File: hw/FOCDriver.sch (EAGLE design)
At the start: 95 parts, among them U1 IX4428N, U2 IX4428N, U3 IX4428N, U4 IRF9389TRPBF, U5 IRF9389TRPBF, U6 IRF9389TRPBF, U7 LM27313XMF, U8 LM358N, U9 LM358N

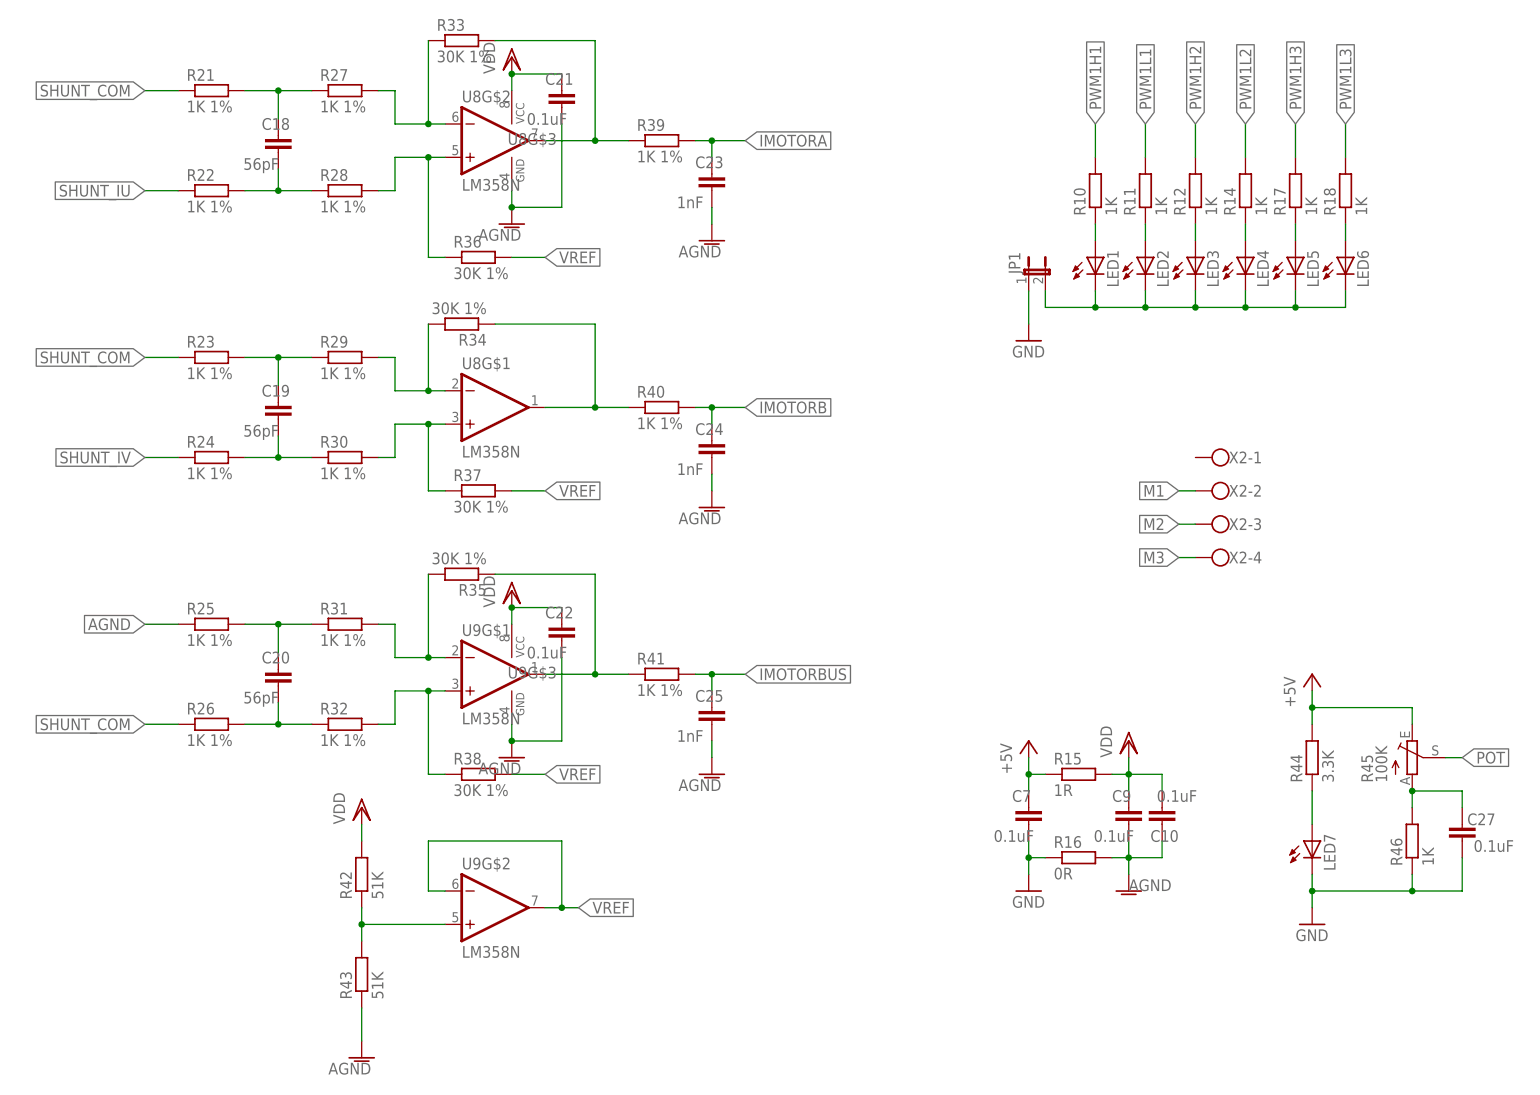
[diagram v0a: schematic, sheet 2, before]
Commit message: layout
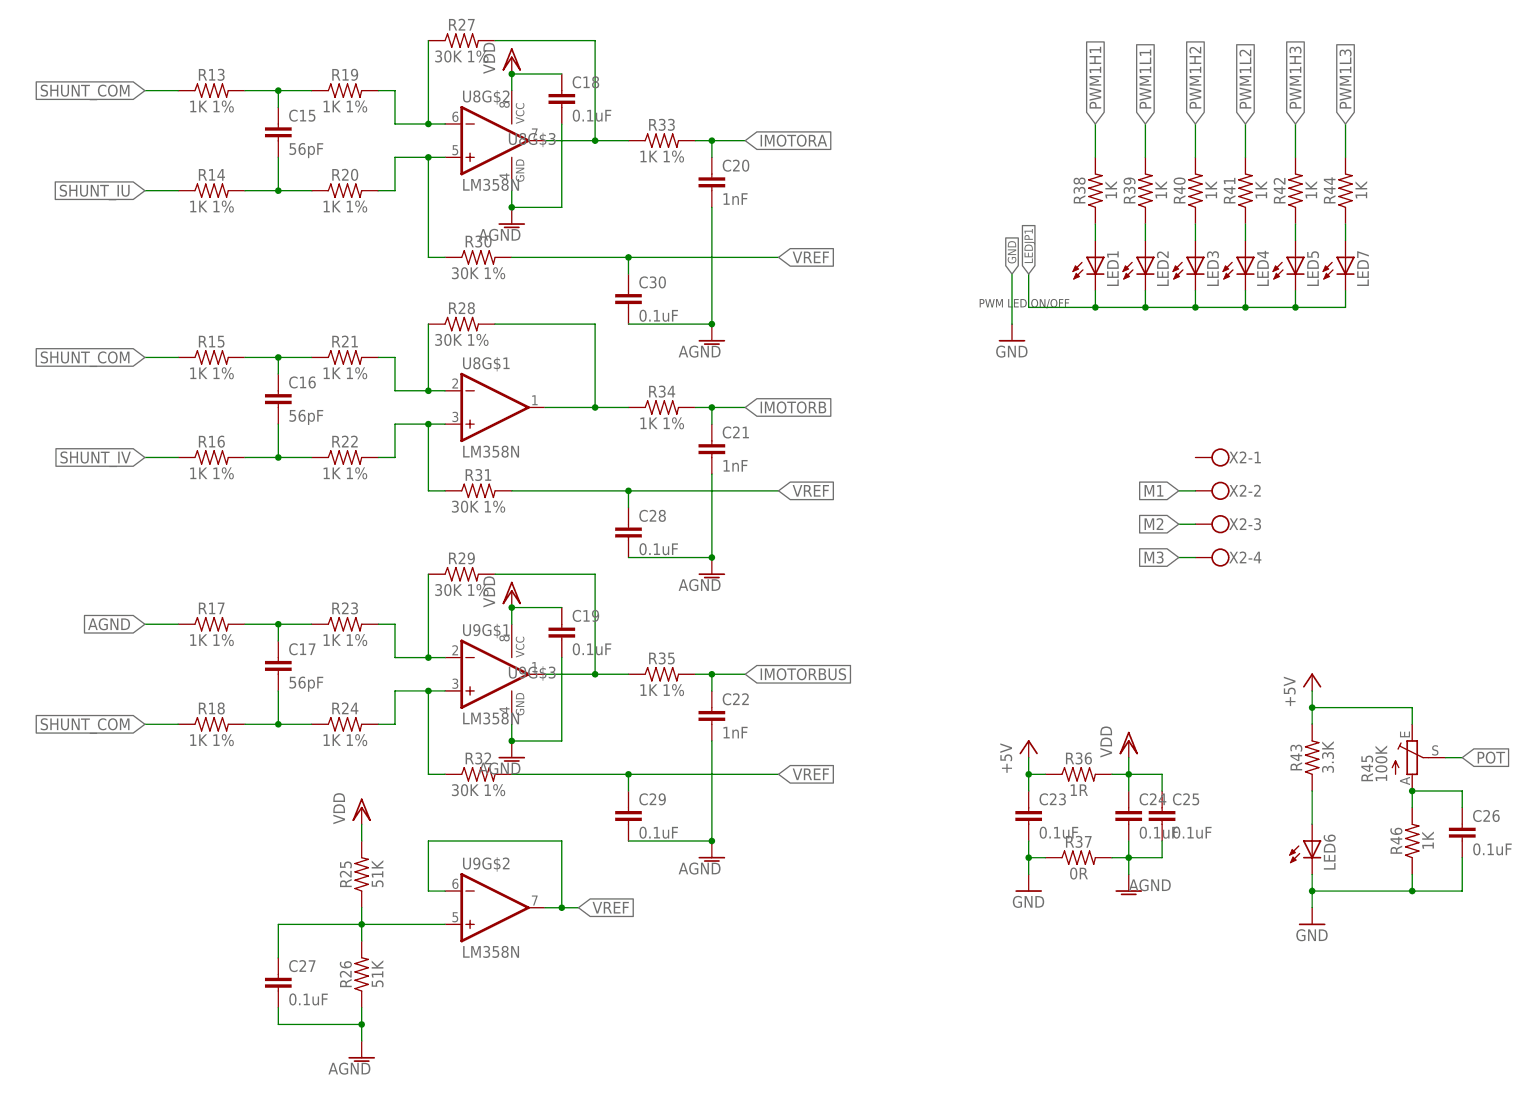
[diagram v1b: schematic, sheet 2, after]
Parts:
- removed J1: (no value), SparkFun-Connectors:CONN_06SILK_FEMALE_PTH
- removed JP1: (no value), jumper:JP1E
- added C26, C28, C29, C30: 0.1uF, SparkFun-Capacitors:1.0UF-0805-25V-10%
- added J4: (no value), SparkFun-Connectors:CONN_08"
- C1, C2, C3: value 1uF -> 1.0uF; device resistor:C-EUC0805 -> SparkFun-Capacitors:1.0UF-0805-25V-10%
- C10, C11, C27, C4, C5, C6, C7, C8, C9: device resistor:C-EUC0805 -> SparkFun-Capacitors:1.0UF-0805-25V-10%
- C12, C21, C22: value 0.1uF -> 1nF; device resistor:C-EUC0805 -> SparkFun-Capacitors:1.0UF-0805-25V-10%
- C13: value 1nF -> 4.7uF; device resistor:C-EUC0805 -> SparkFun-Capacitors:1.0UF-0805-25V-10%
- C14: value 4.7uF -> 470uF; device resistor:C-EUC0805 -> resistor:CPOL-USE2.5-6
- C15, C17: value 0.1uF -> 56pF; device resistor:C-EUC0805 -> SparkFun-Capacitors:1.0UF-0805-25V-10%
- C16: value 470uF -> 56pF; device resistor:CPOL-USE2.5-6 -> SparkFun-Capacitors:1.0UF-0805-25V-10%
- C18, C19: value 56pF -> 0.1uF; device resistor:C-EUC0805 -> SparkFun-Capacitors:1.0UF-0805-25V-10%
- C20: value 56pF -> 1nF; device resistor:C-EUC0805 -> SparkFun-Capacitors:1.0UF-0805-25V-10%
- C23, C24, C25: value 1nF -> 0.1uF; device resistor:C-EUC0805 -> SparkFun-Capacitors:1.0UF-0805-25V-10%
- R1, R3: value 4.7K -> 4.7K; device resistor:R-EU_R0805 -> SparkFun-Resistors:RESISTOR0805
- R10: value 1K -> 51K; device resistor:R-EU_R0805 -> SparkFun-Resistors:RESISTOR0805
- R11: value 1K -> 13.3K; device resistor:R-EU_R0805 -> SparkFun-Resistors:RESISTOR0805
- R12: value 1K -> 118K; device resistor:R-EU_R0805 -> SparkFun-Resistors:RESISTOR0805
- R13: value 51K -> 1K 1%; device resistor:R-EU_R0805 -> SparkFun-Resistors:RESISTOR0805
- R14, R17, R18: value 1K -> 1K 1%; device resistor:R-EU_R0805 -> SparkFun-Resistors:RESISTOR0805
- R15: value 1R -> 1K 1%; device resistor:R-EU_R0805 -> SparkFun-Resistors:RESISTOR0805
- R16: value 0R -> 1K 1%; device resistor:R-EU_R0805 -> SparkFun-Resistors:RESISTOR0805
- R19: value 13.3K -> 1K 1%; device resistor:R-EU_R0805 -> SparkFun-Resistors:RESISTOR0805
- R2, R21, R22, R23, R24, R4, R46, R5, R6: device resistor:R-EU_R0805 -> SparkFun-Resistors:RESISTOR0805
- R20: value 118K -> 1K 1%; device resistor:R-EU_R0805 -> SparkFun-Resistors:RESISTOR0805
- R25, R26: value 1K 1% -> 51K; device resistor:R-EU_R0805 -> SparkFun-Resistors:RESISTOR0805
- R27, R28, R29, R30, R31, R32: value 1K 1% -> 30K 1%; device resistor:R-EU_R0805 -> SparkFun-Resistors:RESISTOR0805
- R33, R34, R35: value 30K 1% -> 1K 1%; device resistor:R-EU_R0805 -> SparkFun-Resistors:RESISTOR0805
- R36: value 30K 1% -> 1R; device resistor:R-EU_R0805 -> SparkFun-Resistors:RESISTOR0805
- R37: value 30K 1% -> 0R; device resistor:R-EU_R0805 -> SparkFun-Resistors:RESISTOR0805
- R38: value 30K 1% -> 1K; device resistor:R-EU_R0805 -> SparkFun-Resistors:RESISTOR0805
- R39, R40, R41: value 1K 1% -> 1K; device resistor:R-EU_R0805 -> SparkFun-Resistors:RESISTOR0805
- R42: value 51K -> 1K; device resistor:R-EU_R0805 -> SparkFun-Resistors:RESISTOR0805
- R43: value 51K -> 3.3K; device resistor:R-EU_R0805 -> SparkFun-Resistors:RESISTOR0805
- R44: value 3.3K -> 1K; device resistor:R-EU_R0805 -> SparkFun-Resistors:RESISTOR0805
- R7, R8, R9: device resistor:R-EU_R2512 -> resistor:R-US_R2512
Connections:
- removed net N$32: JP1.2, LED1.C, LED2.C, LED3.C, LED4.C, LED5.C, LED6.C
- removed net N$38 (its old number): LED6.A, R18.1
- new net LEDJP1: J4.6, LED1.C, LED2.C, LED3.C, LED4.C, LED5.C, LED7.C
- new net N$31: LED6.A, R43.1
- net +12V: now also C1.1, C10.1, C14.+, C2.1, C3.1, C4.1, C5.1, C6.1, C7.1, C9.1, R12.2; no longer C1.2, C14.1, C15.1, C16.+, C17.1, C2.2, C3.2, C4.2, C5.2, C6.2, R20.2
- net +5V: now also C23.1, J2.1, R36.1, R43.2; no longer C7.1, J2.2, R15.1, R44.2
- net AGND: now also C1.2, C10.2, C14.-, C18.2, C19.2, C2.2, C20.2, C27.2, C28.2, C29.2, C3.2, C30.2, C4.2, C5.2, C6.2, C7.2, R11.1, R17.1, R26.1, R37.2, R9.2; no longer C1.1, C10.1, C14.2, C15.2, C16.-, C17.2, C2.1, C23.2, C3.1, C4.1, C5.1, C6.1, R16.2, R19.1, R25.1, R43.1, R9.1
- net AVDD: now also C18.1, C19.1, C24.1, C25.1, R25.2, R36.2; no longer C10.2, C21.1, C22.1, C9.1, R15.2, R42.2
- net GND: now also C23.2, C26.2, J2.2, J4.7, J4.8, LED6.C, R37.1; no longer C27.2, C7.2, J1.6, J2.1, JP1.1, LED7.C, R16.1
- net IMOTORA: now also C20.1, J4.3, R33.2; no longer C23.1, J1.3, R39.2
- net IMOTORB: now also C21.1, J4.2, R34.2; no longer C24.1, J1.2, R40.2
- net IMOTORBUS: now also C22.1, J4.1, R35.2; no longer C25.1, J1.1, R41.2
- net N$1: now also R10.1; no longer R13.1
- net N$11: now also C15.1, R13.2, R19.1; no longer C18.2, R21.2, R27.1
- net N$12: now also C15.2, R14.2, R20.1; no longer C18.1, R22.2, R28.1
- net N$13: now also R19.2, R27.1; no longer R27.2, R33.1
- net N$14: now also C16.1, R15.2, R21.1; no longer C19.2, R23.2, R29.1
- net N$15: now also R20.2, R30.1; no longer R28.2, R36.1
- net N$16: now also R27.2, R33.1; no longer R33.2, R39.1
- net N$17: now also C16.2, R16.2, R22.1; no longer C19.1, R24.2, R30.1
- net N$18: now also C27.1, R25.1, R26.2; no longer R42.1, R43.2
- net N$19: now also R21.2, R28.1; no longer R29.2, R34.2
- net N$2: now also R10.2; no longer R13.2
- net N$20: now also R22.2, R31.1; no longer R30.2, R37.1
- net N$21: now also R28.2; no longer R40.1
- net N$22: now also C17.1, R17.2, R23.1; no longer C20.2, R25.2, R31.1
- net N$23: now also C17.2, R18.2, R24.1; no longer C20.1, R26.2, R32.1
- net N$24: now also R23.2, R29.1; no longer R31.2, R35.2
- net N$25: now also R24.2, R32.1; no longer R32.2, R38.1
- net N$26: now also R29.2; no longer R41.1
- net N$29: now also C26.1; no longer C27.1
- net N$33: now also R38.1; no longer R10.1
- net N$34: now also R39.1; no longer R11.1
- net N$35: now also R40.1; no longer R12.1
- net N$36: now also R41.1; no longer R14.1
- net N$37: now also R42.1; no longer R17.1
- net N$4: now also R11.2, R12.1; no longer R19.2, R20.1
- net POT: now also J4.5; no longer J1.5
- net PWM1H1: now also R38.2; no longer R10.2
- net PWM1H2: now also R40.2; no longer R12.2
- net PWM1H3: now also R42.2; no longer R17.2
- net PWM1L1: now also R39.2; no longer R11.2
- net PWM1L2: now also R41.2; no longer R14.2
- net PWM1L3: now also R44.2; no longer R18.2
- net SHUNT_COM: now also R13.1, R15.1, R18.1, R7.2, R8.2, R9.1; no longer R21.1, R23.1, R26.1, R7.1, R8.1, R9.2
- net SHUNT_IU: now also R14.1, R7.1; no longer R22.1, R7.2
- net SHUNT_IV: now also R16.1, R8.1; no longer R24.1, R8.2
- net VREF: now also C28.1, C29.1, C30.1, R30.2, R31.2, R32.2; no longer R36.2, R37.2, R38.2
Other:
- note added: "PWM LED ON/OFF"
- moved on the sheet: C1, C12, C13, C18, C19, C2, C20, C21, C22, C23, C24, C25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
